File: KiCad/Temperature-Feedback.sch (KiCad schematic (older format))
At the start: 8 parts, among them U2 MCP41050, U3 MCP9700A, U4 MCP617

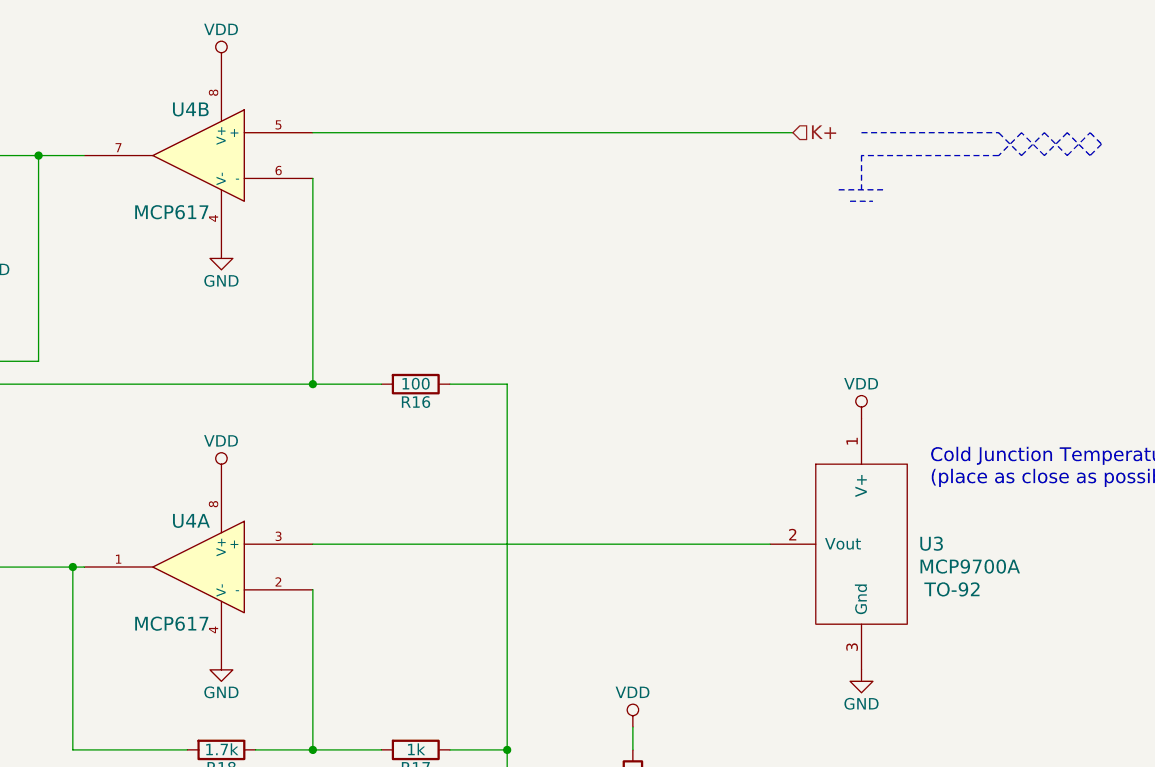
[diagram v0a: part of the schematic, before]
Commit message: IC BOM and footprints complete
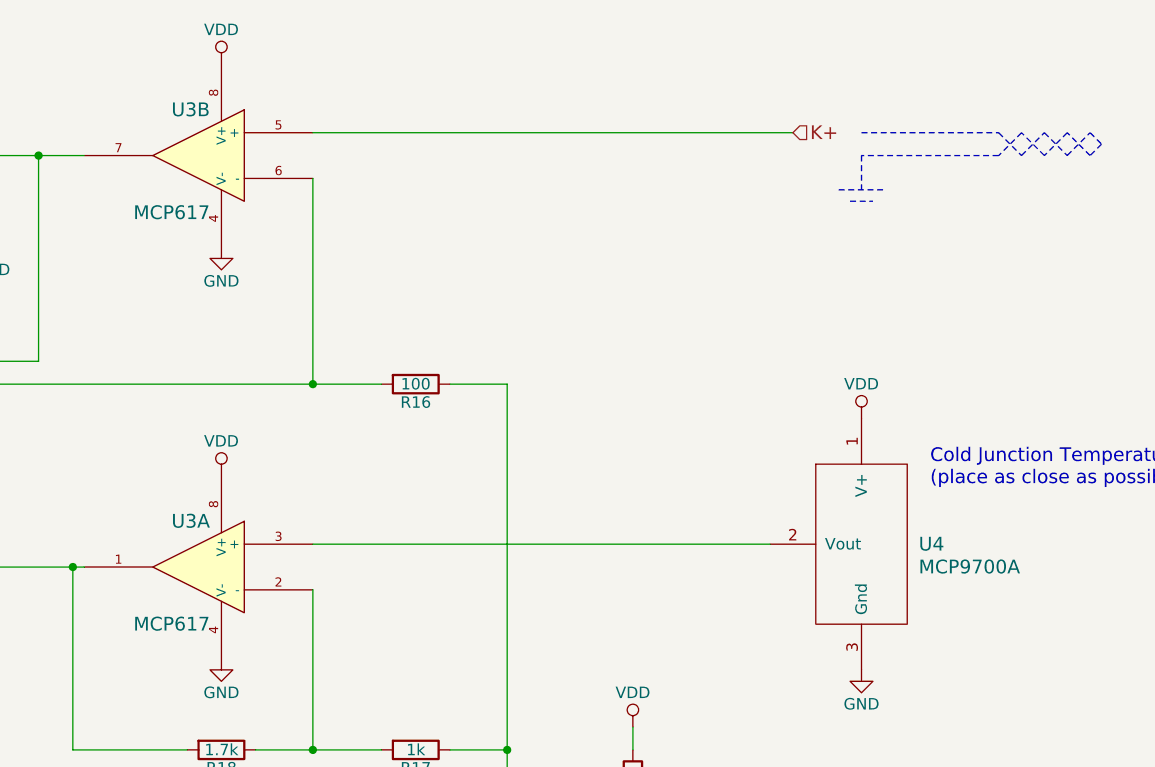
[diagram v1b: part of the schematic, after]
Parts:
- U2, U4: footprint (none) -> Easy-PCB-footprints:DIP-8
- U4: renamed from U3; footprint TO-92 -> Easy-PCB-footprints:TO-92
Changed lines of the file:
@@
 P 5800 3900
 AR Path="/564E7160" Ref="U4"  Part="1"
-AR Path="/564E6B87/564E7160" Ref="U4"  Part="1"
-F 0 "U4" H 5750 4100 60  0000 L CNN
+AR Path="/564E6B87/564E7160" Ref="U3"  Part="1"
+F 0 "U3" H 5750 4100 60  0000 L CNN
 F 1 "MCP617" H 5750 3650 60  0000 L CNN
-F 2 "" H 5800 3900 60  0001 C CNN
+F 2 "Easy-PCB-footprints:DIP-8" H 5800 3900 60  0001 C CNN
 F 3 "" H 5800 3900 60  0000 C CNN
 	1    5800 3900
@@
 P 5800 2100
 AR Path="/564E743F" Ref="U4"  Part="2"
-AR Path="/564E6B87/564E743F" Ref="U4"  Part="2"
-F 0 "U4" H 5750 2300 60  0000 L CNN
+AR Path="/564E6B87/564E743F" Ref="U3"  Part="2"
+F 0 "U3" H 5750 2300 60  0000 L CNN
 F 1 "MCP617" H 5750 1850 60  0000 L CNN
-F 2 "" H 5800 2100 60  0001 C CNN
+F 2 "Easy-PCB-footprints:DIP-8" H 5800 2100 60  0001 C CNN
 F 3 "" H 5800 2100 60  0000 C CNN
 	2    5800 2100
@@
 F 0 "U2" H 4450 3400 60  0000 C CNN
 F 1 "MCP41050" H 4450 2700 60  0000 C CNN
-F 2 "" H 4450 3050 60  0001 C CNN
+F 2 "Easy-PCB-footprints:DIP-8" H 4450 3050 60  0001 C CNN
 F 3 "" H 4450 3050 60  0000 C CNN
 	1    4450 3050
@@
 $EndComp
 $Comp
-L MCP9700A U3
+L MCP9700A U4
 U 1 1 56880F29
 P 8700 3800
-F 0 "U3" H 8950 3800 60  0000 L CNN
+F 0 "U4" H 8950 3800 60  0000 L CNN
 F 1 "MCP9700A" H 8950 3700 60  0000 L CNN
-F 2 "TO-92" H 9100 3600 60  0000 C CNN
+F 2 "Easy-PCB-footprints:TO-92" H 9100 3600 60  0001 C CNN
 F 3 "" H 8700 3800 60  0000 C CNN
 	1    8700 3800
